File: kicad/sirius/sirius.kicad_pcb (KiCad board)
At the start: 4 copper layers, 42.1 x 65.5 mm, 60 parts, among them J1 IPEX_MHF1, J2 Power In, J3 Screw_Terminal, Q1 Q_PMOS_GSD, Q2 Q_NMOS_GSD, Q3 Q_NMOS_GSD, U1 Power_Connector, U2 AP63301WU-7, U3 RFM95W-915S2, U4 LC29H (DA), U5 Pi Zero 2W

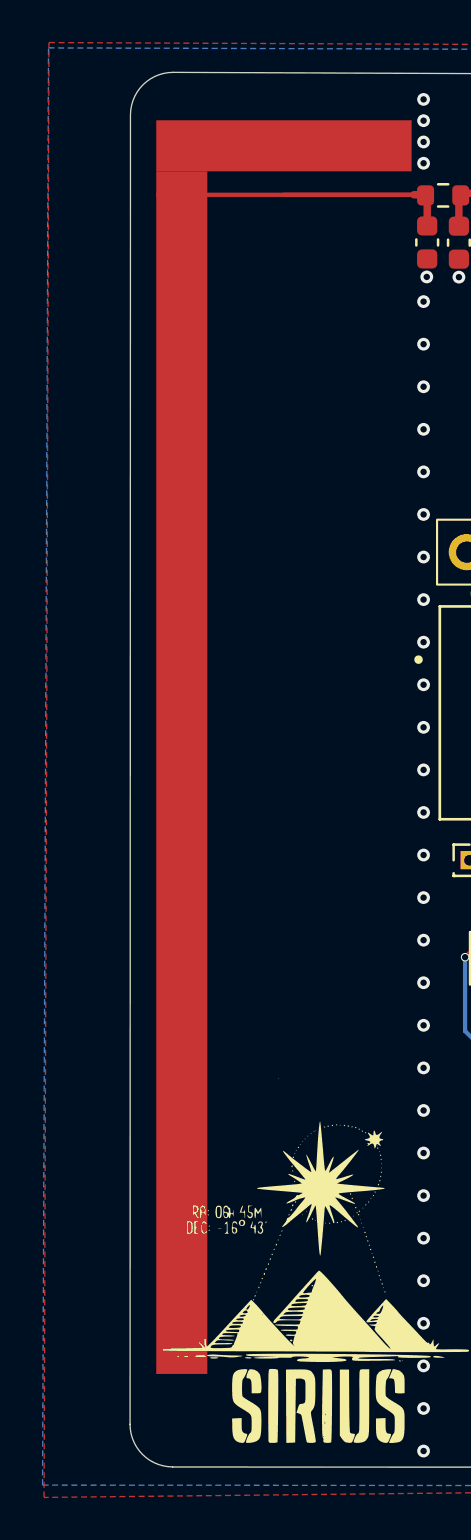
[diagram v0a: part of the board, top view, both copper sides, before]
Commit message: Add code for rocket and ground station
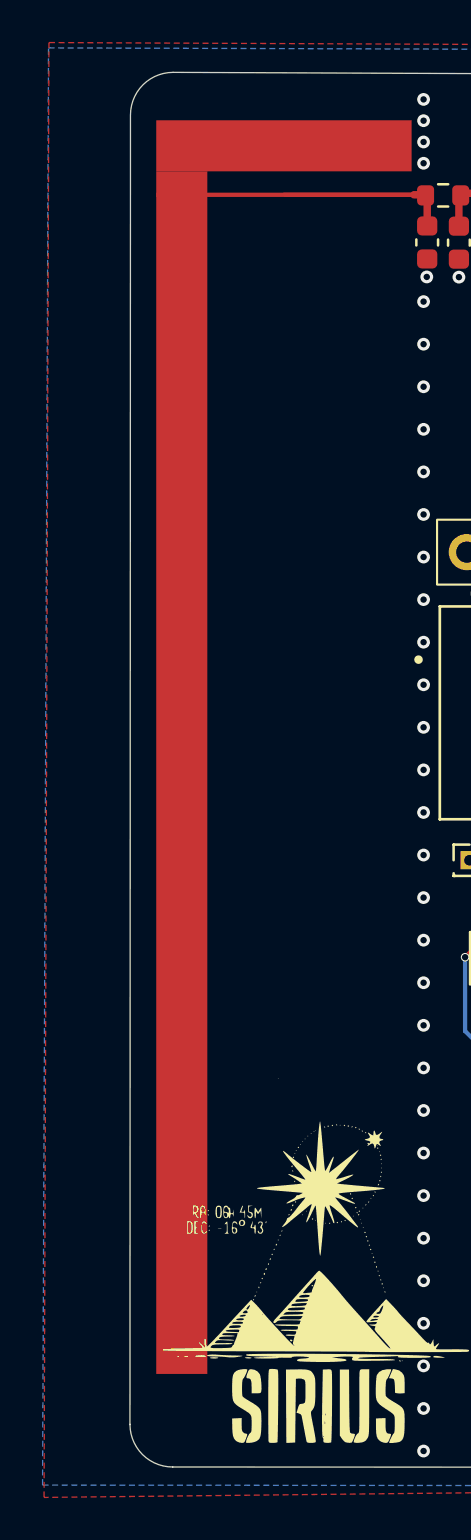
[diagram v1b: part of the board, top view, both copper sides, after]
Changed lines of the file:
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@@
 	)
 	(gr_line
-		(start 113.07 129.815786)
+		(start 113.065796 129.815786)
 		(end 113.09 68.31)
 		(stroke
@@
 	)
 	(gr_arc
-		(start 115.07 131.815786)
-		(mid 113.655786 131.23)
-		(end 113.07 129.815786)
+		(start 115.074214 131.82)
+		(mid 113.654299 131.234471)
+		(end 113.065796 129.815786)
 		(stroke
 			(width 0.05)
